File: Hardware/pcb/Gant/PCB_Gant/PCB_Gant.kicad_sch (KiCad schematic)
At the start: 4 parts, among them SW1 SW_SPST, U1 STM32G431KBTx

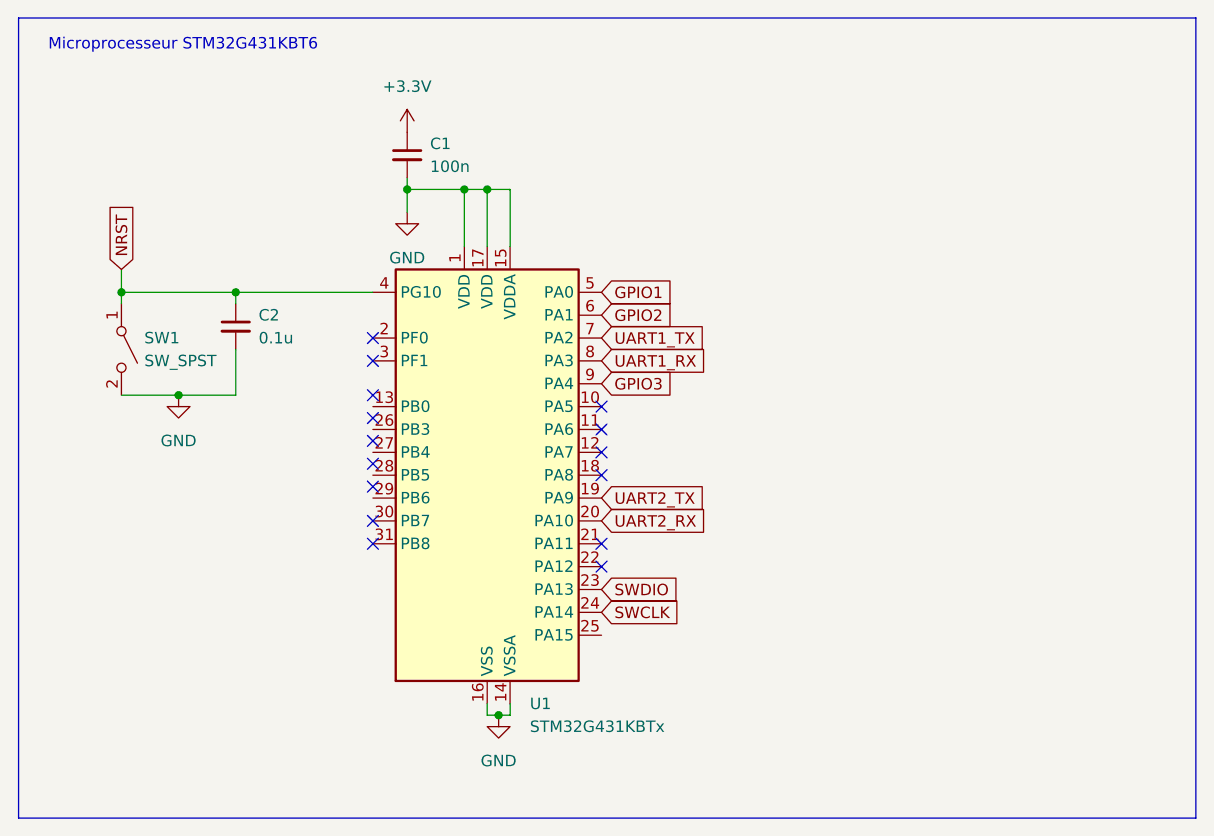
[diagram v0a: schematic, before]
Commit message: modifications on schematic
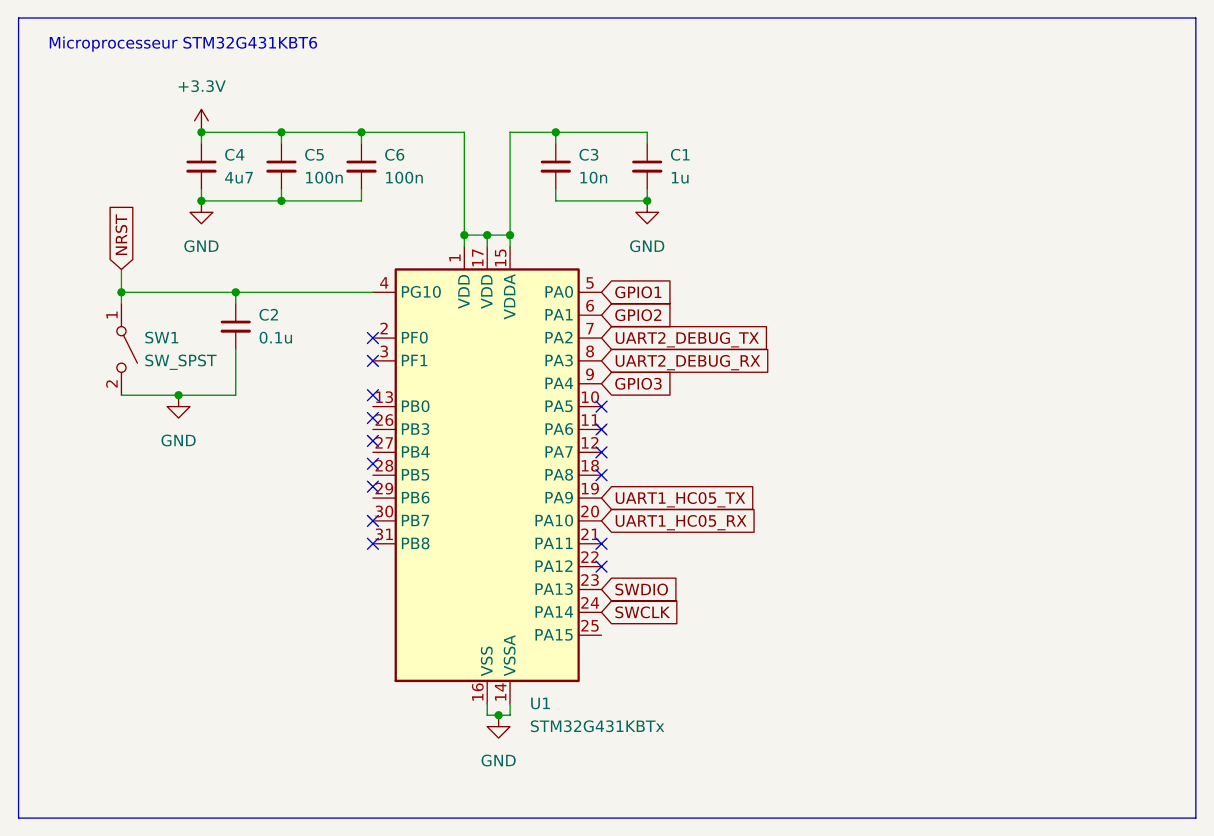
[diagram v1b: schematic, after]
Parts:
- added C3: 10n, symbol Device:C_Small
- added C4: 4u7, symbol Device:C_Small
- added C5, C6: 100n, symbol Device:C_Small
- C1: value 100n -> 1u
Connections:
- net +3.3V: now also U1.1 (VDD), U1.15 (VDDA), U1.17 (VDD), C3.1, C4.1, C5.1, C6.1
- net GND: now also C3.2, C4.2, C5.2, C6.2; no longer U1.1 (VDD), U1.15 (VDDA), U1.17 (VDD)
- net UART1_RX renamed UART2_DEBUG_RX
- net UART1_TX renamed UART2_DEBUG_TX
- net UART2_RX renamed UART1_HC05_RX
- net UART2_TX renamed UART1_HC05_TX
